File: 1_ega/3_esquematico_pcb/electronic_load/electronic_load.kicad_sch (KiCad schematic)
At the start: 39 parts, among them J1 Encoder, J10 VCC, J11 LOAD, J12 FAN, J2 LCD_I2C, J3 GND, J4 MOS_GATE, J5 Isense, J6 Vload_LPF, J7 5V, J8 MOS_LPF, J9 TEMP_DIODE, Q1 IRF540N, Q2 2n2222, SW1 BTN_MENU, SW2 BTN_STOP, U1 TL084

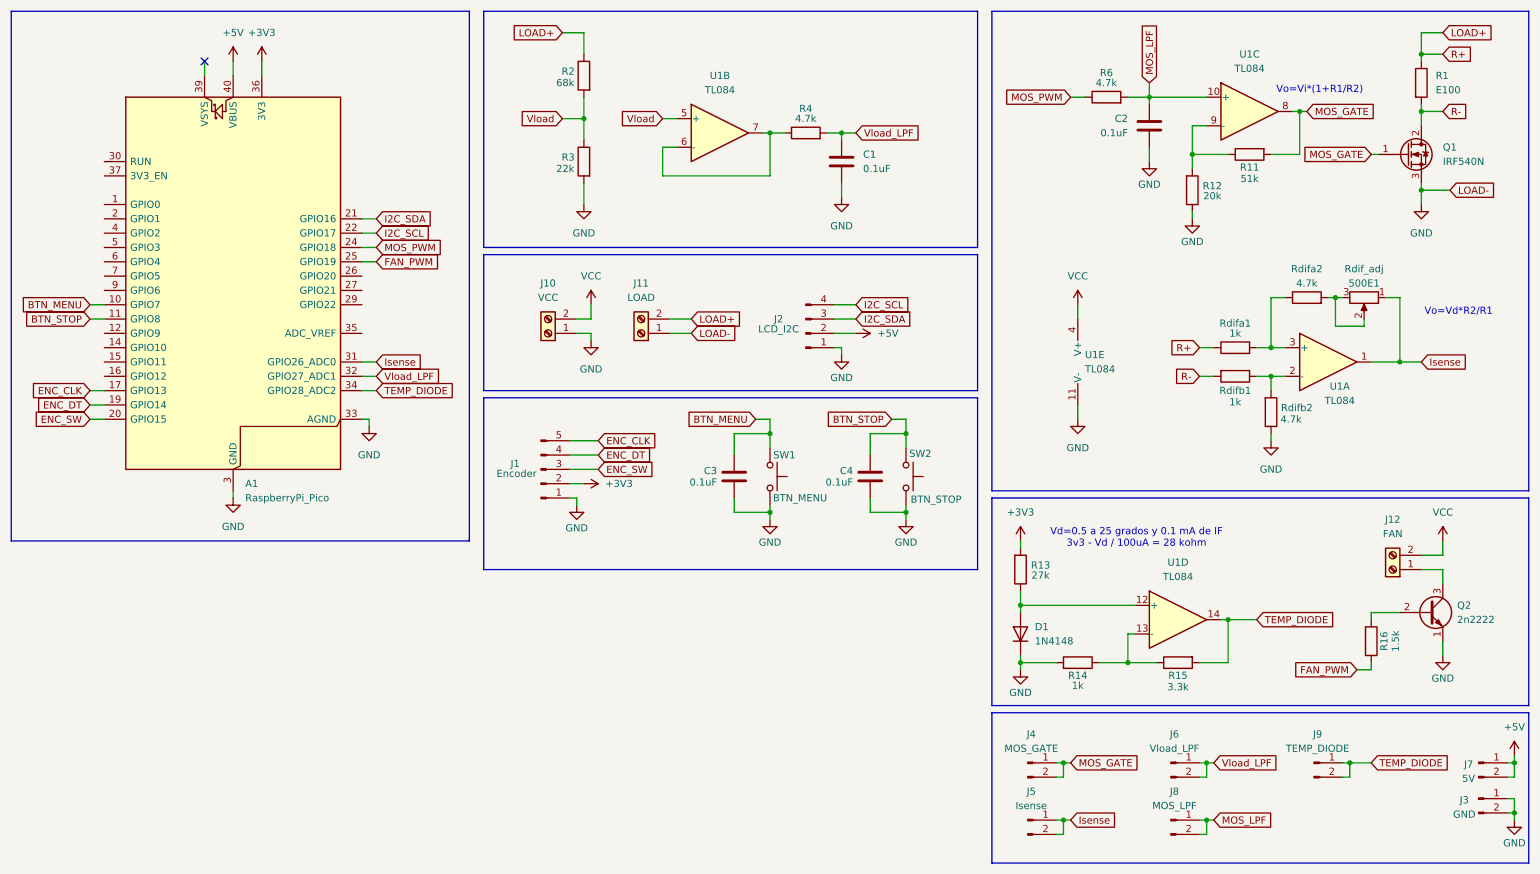
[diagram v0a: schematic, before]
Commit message: add: diagrama de conexiones y modificar firmware
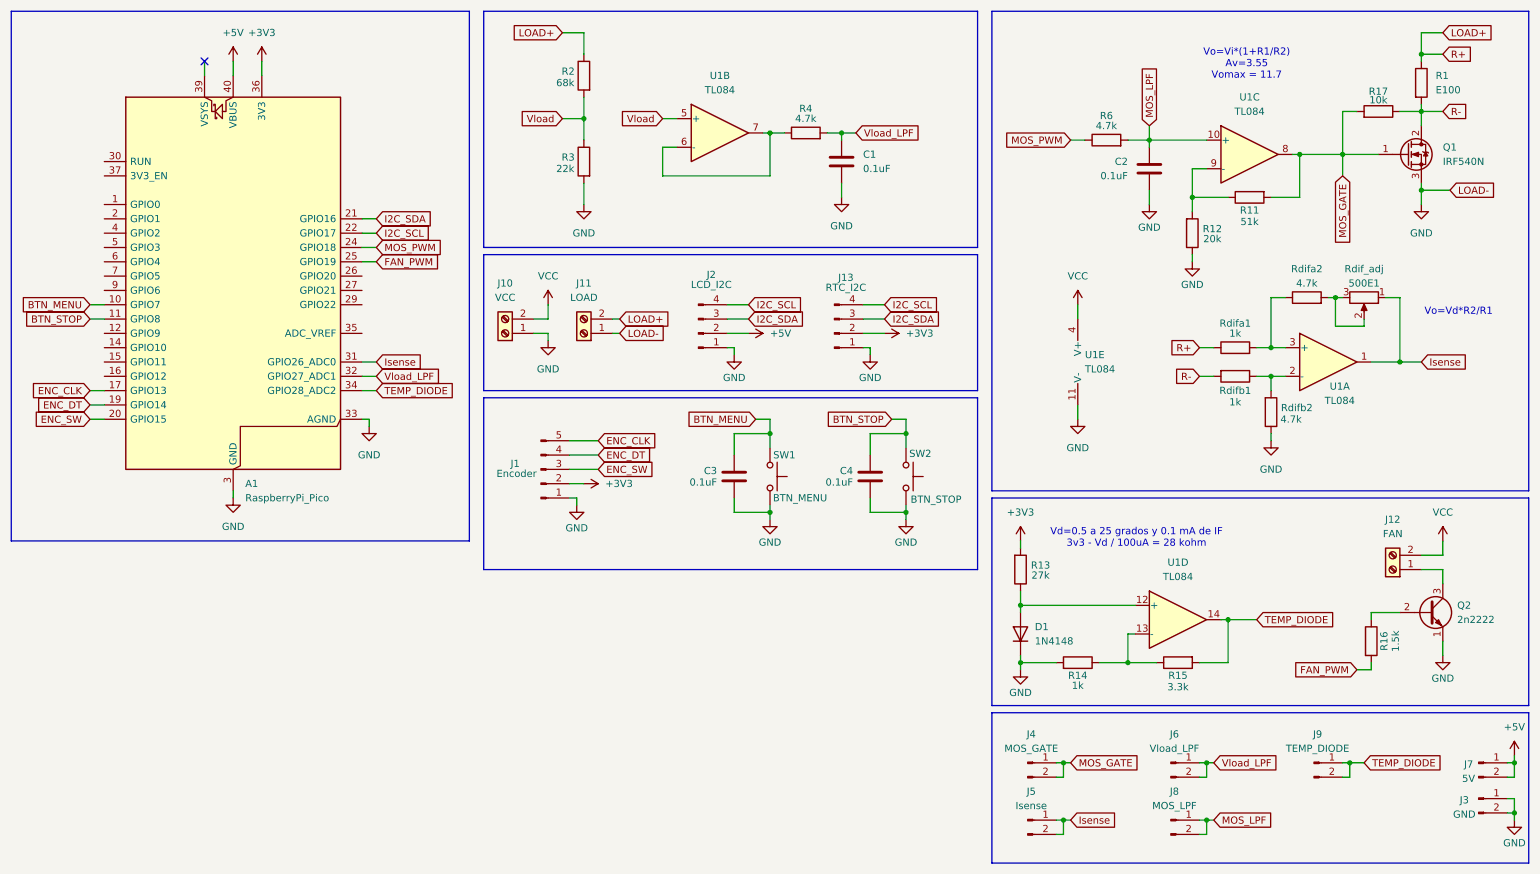
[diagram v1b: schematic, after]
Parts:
- added J13: RTC_I2C, Connector_PinSocket_2.54mm:PinSocket_1x04_P2.54mm_Vertical, symbol Connector:Conn_01x04_Pin
- added R17: 10k, Resistor_THT:R_Axial_DIN0207_L6.3mm_D2.5mm_P10.16mm_Horizontal, symbol Device:R
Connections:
- net +3V3: now also J13.2 (Pin_2)
- net GND: now also J13.1 (Pin_1)
- net I2C_SCL: now also J13.4 (Pin_4)
- net I2C_SDA: now also J13.3 (Pin_3)
- net MOS_GATE: now also R17.2
- net R-: now also R17.1
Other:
- note added: "Vo=Vi*(1+R1/R2) Av=3.55 Vomax = 11.7"
- note removed: "Vo=Vi*(1+R1/R2)"
- moved on the sheet: C2, J10, J11, J2, R11, R12, R6, U1C
